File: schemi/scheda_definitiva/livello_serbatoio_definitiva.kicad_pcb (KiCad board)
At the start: 2 copper layers, 83 x 72 mm, 49 parts, among them J1 USB_B, J2 BTN_LED_GROUP, J3 CONN_LCD, J4 CONN_US, J5 ICSP, J6 Exp_Analog_2, J7 Exp_Analog, SW1 SW_RST, U1 FT232RL, U2 ATmega328P-PU, U3 USBLC6-2SC6, Y1 16MHz

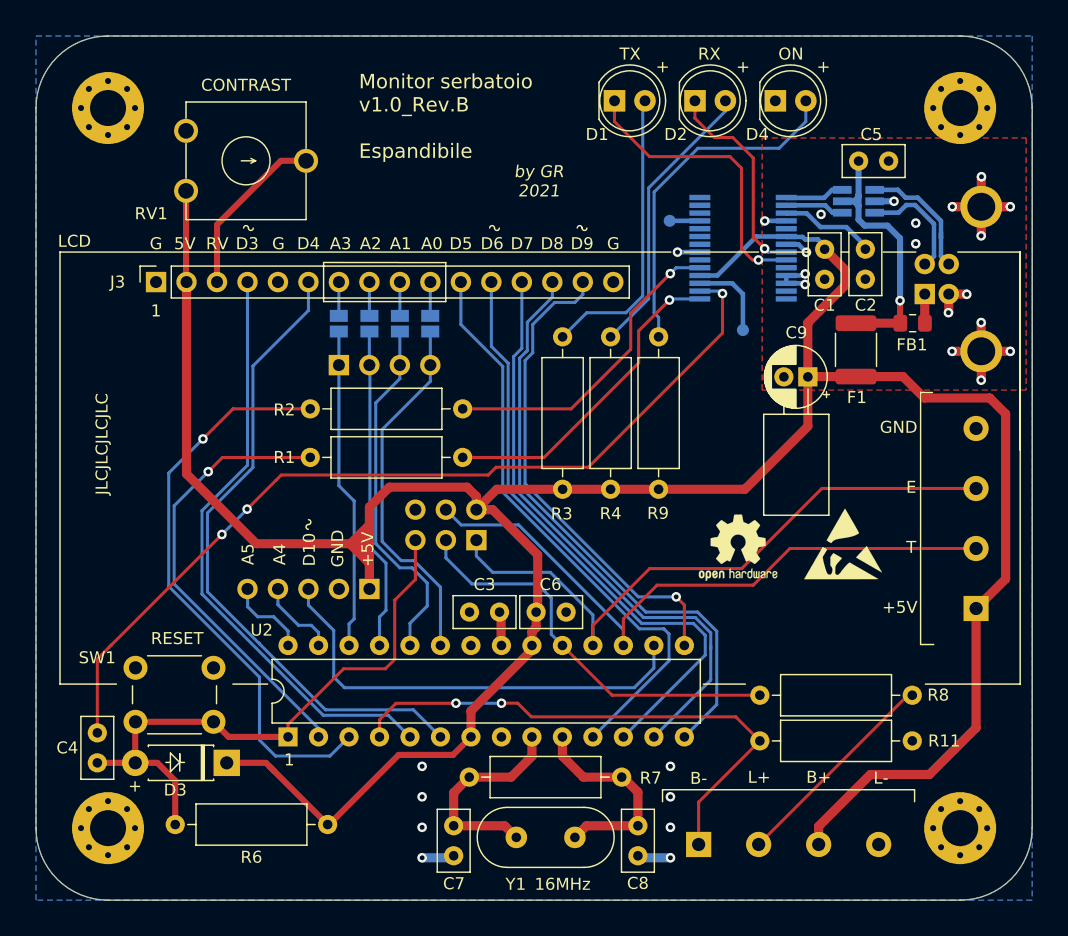
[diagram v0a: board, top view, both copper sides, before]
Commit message: modifiche scheda definitiva (rev. C)
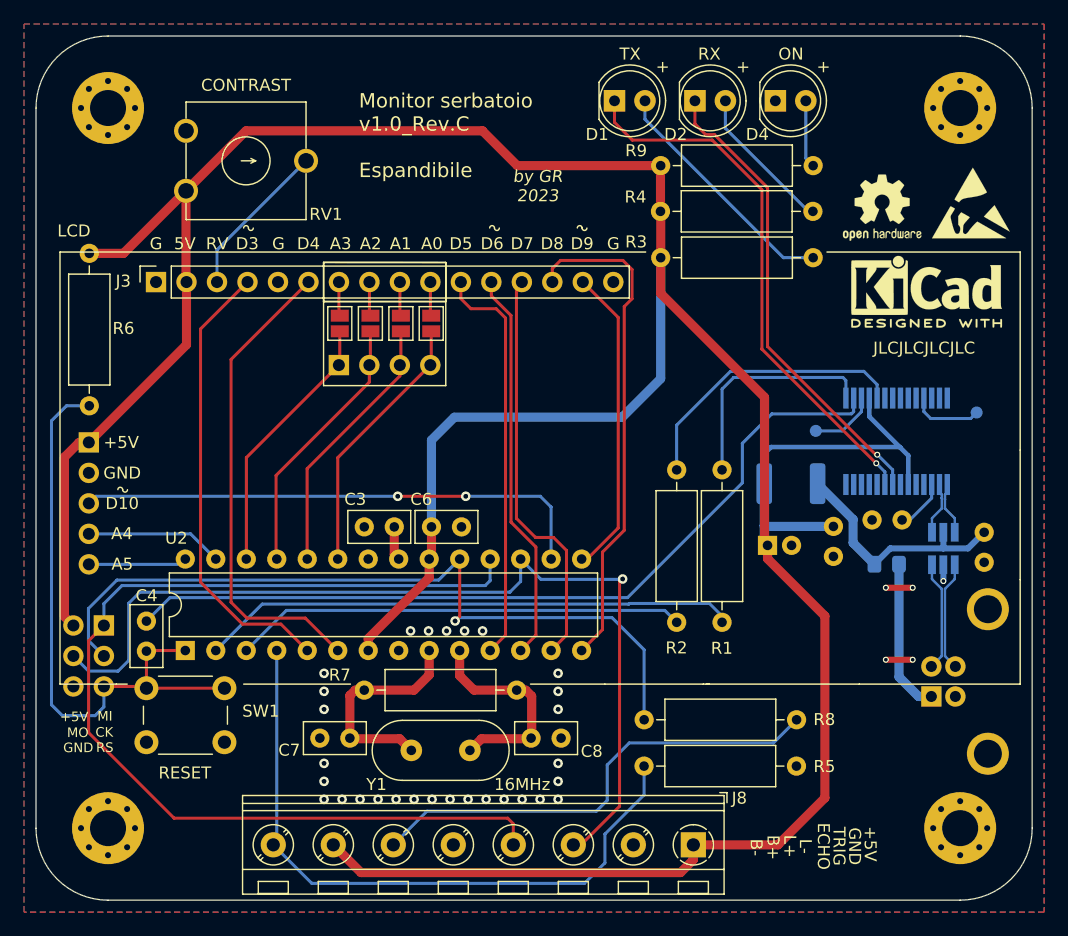
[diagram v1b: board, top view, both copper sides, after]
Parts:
- removed D3: 1N4700, Diode_THT:D_DO-41_SOD81_P7.62mm_Horizontal
- removed J2: BTN_LED_GROUP, simboli_custom:TerminalBlock_RND_205-00047_1x04_P5.00mm_Horizontal
- removed J4: CONN_US, simboli_custom:TerminalBlock_RND_205-00047_1x04_P5.00mm_Horizontal
- removed R11: 10k, Resistor_THT:R_Axial_DIN0309_L9.0mm_D3.2mm_P12.70mm_Horizontal
- added J8: Ext_connections, TerminalBlock_RND:TerminalBlock_RND_205-00051_1x08_P5.00mm_Horizontal, F.Cu at (141.8, 135.4)
- added R5: 10k, Resistor_THT:R_Axial_DIN0309_L9.0mm_D3.2mm_P12.70mm_Horizontal, F.Cu at (137.7, 128.8)
- added REF**: KiCad-Logo2_5mm_SilkScreen, Symbol:KiCad-Logo2_5mm_SilkScreen, F.Cu at (161.2, 89.3)
- C1, C2, C5, C9, F1, FB1: moved to B.Cu
- JP1, JP2, JP3, JP4: moved to F.Cu
- moved R6 51.6 mm to (91.4, 86.1), turned to -90 degrees
- moved R1 37.0 mm to (144.2, 116.8), turned to 90 degrees
- moved R2 35.3 mm to (140.4, 116.8), turned to 90 degrees
- moved C5 34.4 mm to (166.0, 111.8), turned to 90 degrees
- moved J1 33.5 mm to (161.6, 123.0)
- moved J5 31.8 mm to (92.7, 117.1), turned to 180 degrees
- moved REF** 30.8 mm to (157.5, 82.3)
- moved REF** 30.3 mm to (164.9, 81.9)
- moved TP2 30.1 mm to (165.4, 99.4), turned to 180 degrees
- moved U3 29.8 mm to (162.6, 110.7), turned to 90 degrees
- moved J7 26.4 mm to (91.4, 101.9), turned to 180 degrees
- moved R4 23.5 mm to (139.0, 82.6), turned to 0 degrees
- moved C1 23.1 mm to (153.4, 111.4)
- moved C2 22.8 mm to (159.2, 108.3), turned to 180 degrees
- moved R3 21.0 mm to (139.1, 86.5), turned to 0 degrees
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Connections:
- U1 pad 10: Net-(U1-Pad10) -> unconnected-(U1-DCD-Pad10)
- U1 pad 12: Net-(U1-Pad12) -> unconnected-(U1-CBUS4-Pad12)
- U1 pad 13: Net-(U1-Pad13) -> unconnected-(U1-CBUS2-Pad13)
- U1 pad 14: Net-(U1-Pad14) -> unconnected-(U1-CBUS3-Pad14)
- U1 pad 19: Net-(U1-Pad19) -> unconnected-(U1-~{RESET}-Pad19)
- U1 pad 27: Net-(U1-Pad27) -> unconnected-(U1-OSCI-Pad27)
- U1 pad 28: Net-(U1-Pad28) -> unconnected-(U1-OSCO-Pad28)
- U1 pad 6: Net-(U1-Pad6) -> unconnected-(U1-RI-Pad6)
- U1 pad 9: Net-(U1-Pad9) -> unconnected-(U1-DCR-Pad9)
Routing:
- net VDD: track 240.9 -> 287.8 mm
- net GND: track 39.2 -> 5.82 mm, vias 27 -> 34
- net D12: track 53.9 -> 86.6 mm
- net D13: track 34.1 -> 65.6 mm, vias 0 -> 1
- net D11: track 54.3 -> 79.0 mm, vias 0 -> 1
- net Net-(D4-A): track 29.0 -> 5.65 mm
- net Net-(D2-K): track 17.6 -> 39.3 mm
- net Net-(J8-Pin_6): track 18.2 -> 39.6 mm
- net Net-(D1-K): track 24.8 -> 45.2 mm
- net D6: track 50.6 -> 32.8 mm
- net D7: track 49.7 -> 34.0 mm
- net D5: track 48.9 -> 34.0 mm
- net BLA: track 40.6 -> 25.8 mm, vias 1 -> 0
- net D4: track 53.9 -> 39.9 mm
- net D3: track 49.8 -> 37.9 mm
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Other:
- net class Default removed
- board text added: "ECHO"
- board text added: "Monitor serbatoio v1.0_Rev.C Espandibile"
- board text added: "TRIG"
- board text added: "by GR 2023"
- board text removed: "1"
- board text removed: "BTN"
- board text removed: "E"
- board text removed: "Monitor serbatoio v1.0_Rev.B Espandibile"
- board text removed: "SENS"
- board text removed: "T"
- board text removed: "by GR 2021"
